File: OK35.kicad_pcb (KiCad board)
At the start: 2 copper layers, 133.3 x 116.2 mm, 78 parts, among them SW1 SW_SPST, SW10 SW_SPST, SW11 SW_SPST, SW12 SW_SPST, SW13 SW_SPST, SW14 SW_SPST, SW15 SW_SPST, SW16 SW_SPST, SW17 SW_SPST, SW18 SW_SPST, SW19 SW_SPST, SW2 SW_SPST, SW20 SW_SPST, SW21 SW_SPST, SW22 SW_SPST, SW23 SW_SPST, SW24 SW_SPST, SW25 SW_SPST, SW26 SW_SPST, SW27 SW_SPST, SW28 SW_SPST, SW29 SW_SPST, SW3 SW_SPST, SW30 SW_SPST, SW31 SW_SPST, SW32 SW_SPST, SW33 SW_SPST, SW34 SW_SPST, SW35 SW_SPST, SW4 SW_SPST, SW5 SW_SPST, SW6 SW_SPST, SW7 SW_SPST, SW8 SW_SPST, SW9 SW_SPST, U1 TRRS, U2 ProMicro

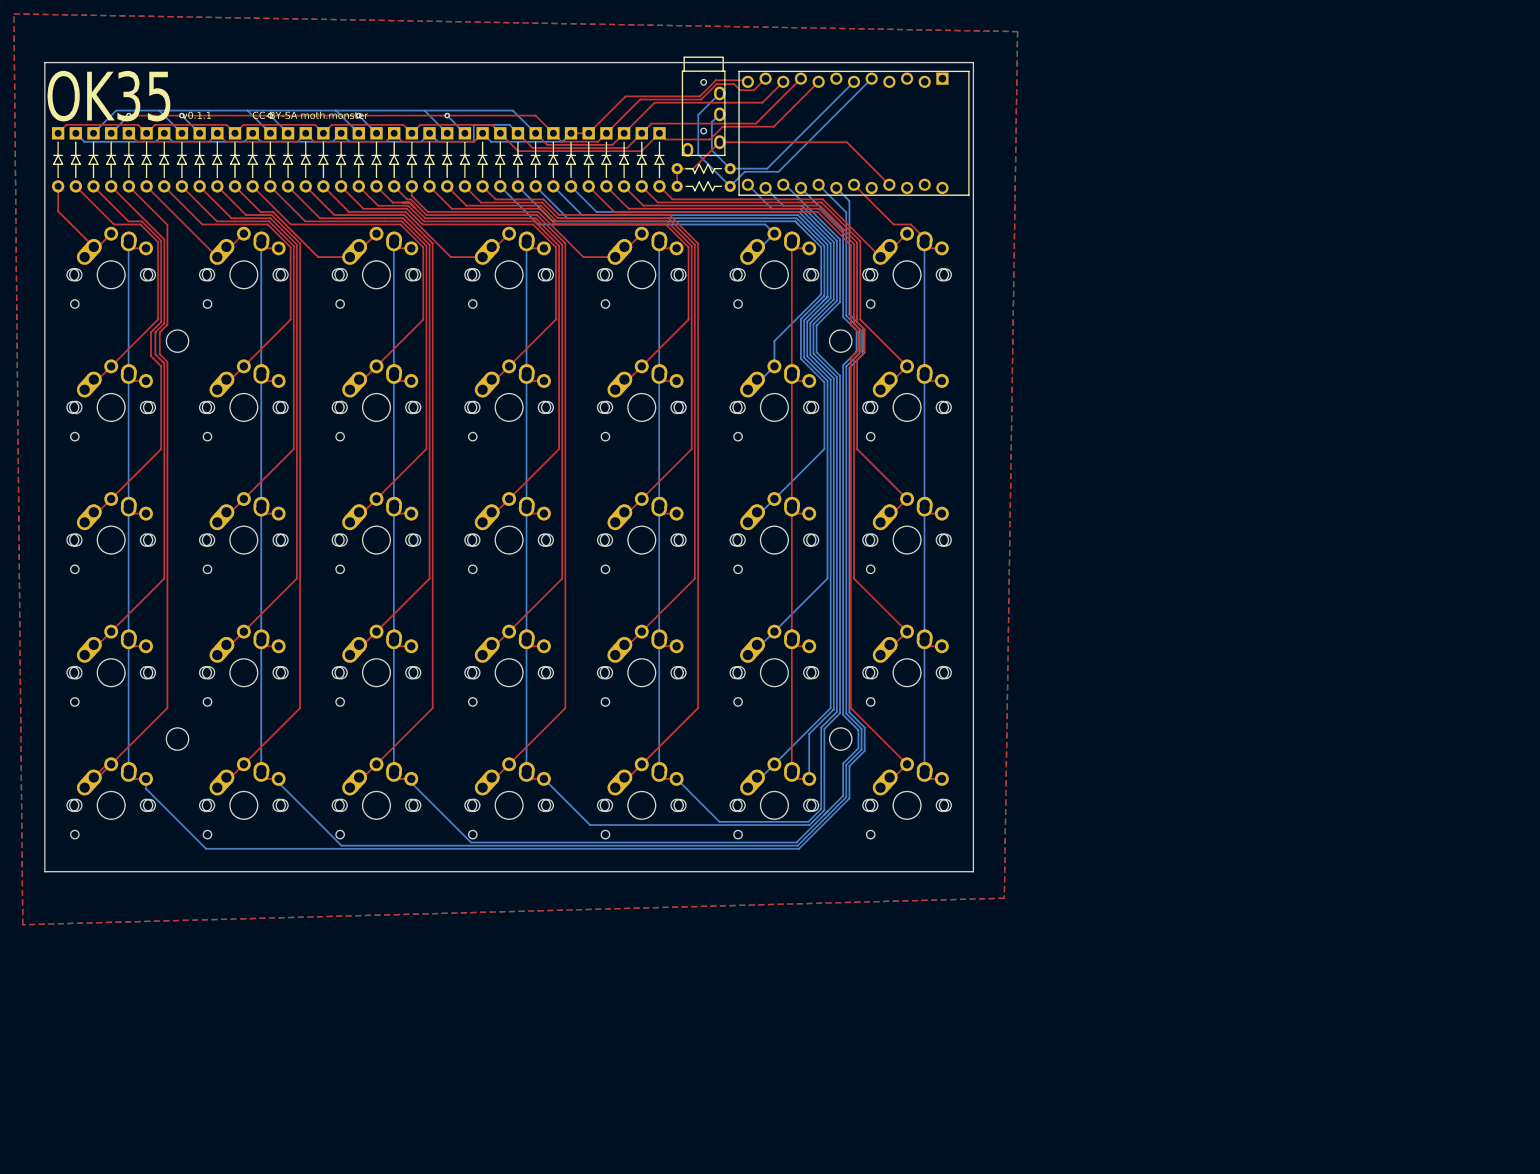
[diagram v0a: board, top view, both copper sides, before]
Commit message: cleanup some stuff
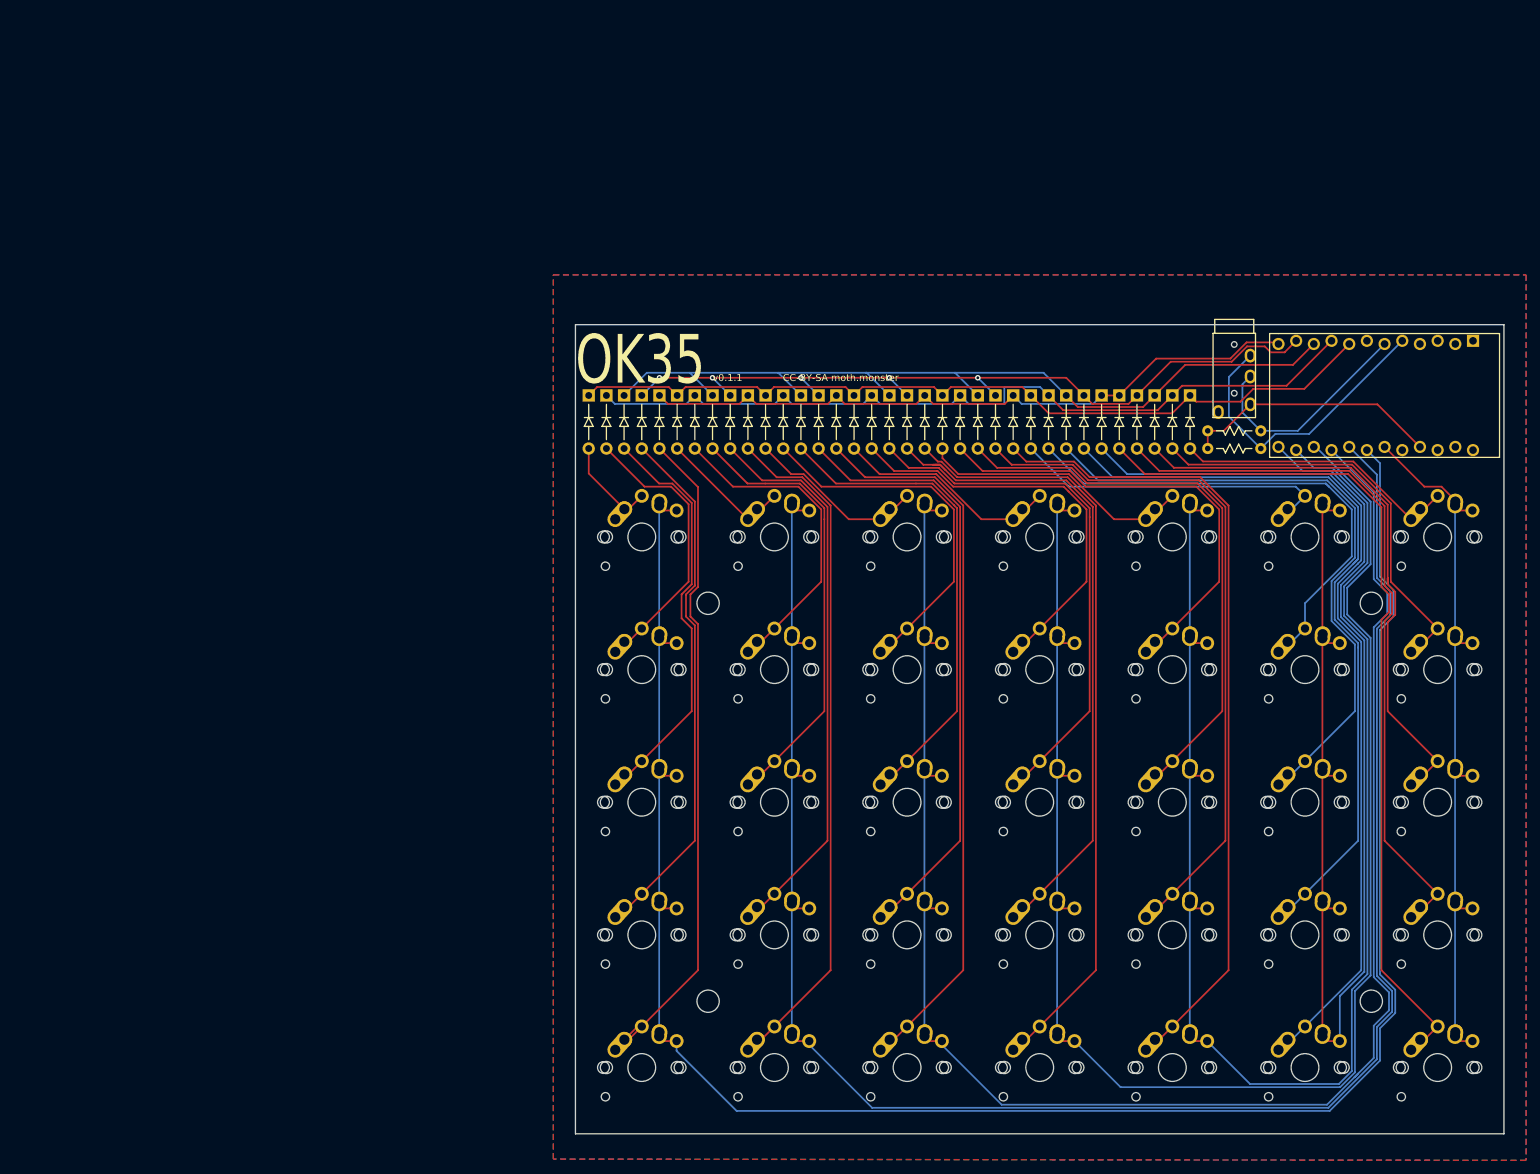
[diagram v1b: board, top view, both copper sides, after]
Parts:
- moved R1 85.0 mm to (177.8, 50.4)
- moved R2 85.0 mm to (177.8, 47.8)
- moved REF** 85.0 mm to (193.7, 72.6)
- moved SW18 85.0 mm to (146.1, 101.2)
- moved SW25 85.0 mm to (146.1, 120.2)
- moved SW32 85.0 mm to (146.1, 139.2)
- moved D1 85.0 mm to (86.4, 46.5)
- moved D11 85.0 mm to (127.0, 46.5)
- moved D13 85.0 mm to (152.4, 46.5)
- moved D14 85.0 mm to (170.2, 46.5)
- moved D15 85.0 mm to (91.4, 46.5)
- moved D16 85.0 mm to (104.1, 46.5)
- moved D17 85.0 mm to (116.8, 46.5)
- moved D19 85.0 mm to (142.2, 46.5)
- moved D2 85.0 mm to (99.1, 46.5)
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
